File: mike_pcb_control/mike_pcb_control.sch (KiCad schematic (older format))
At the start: 5 parts, among them J1 Conn_01x06_Male, J4 Raspberry_Pi_2_3, U3 LLC-4channel, U4 Adafruit_Feather_Pinout

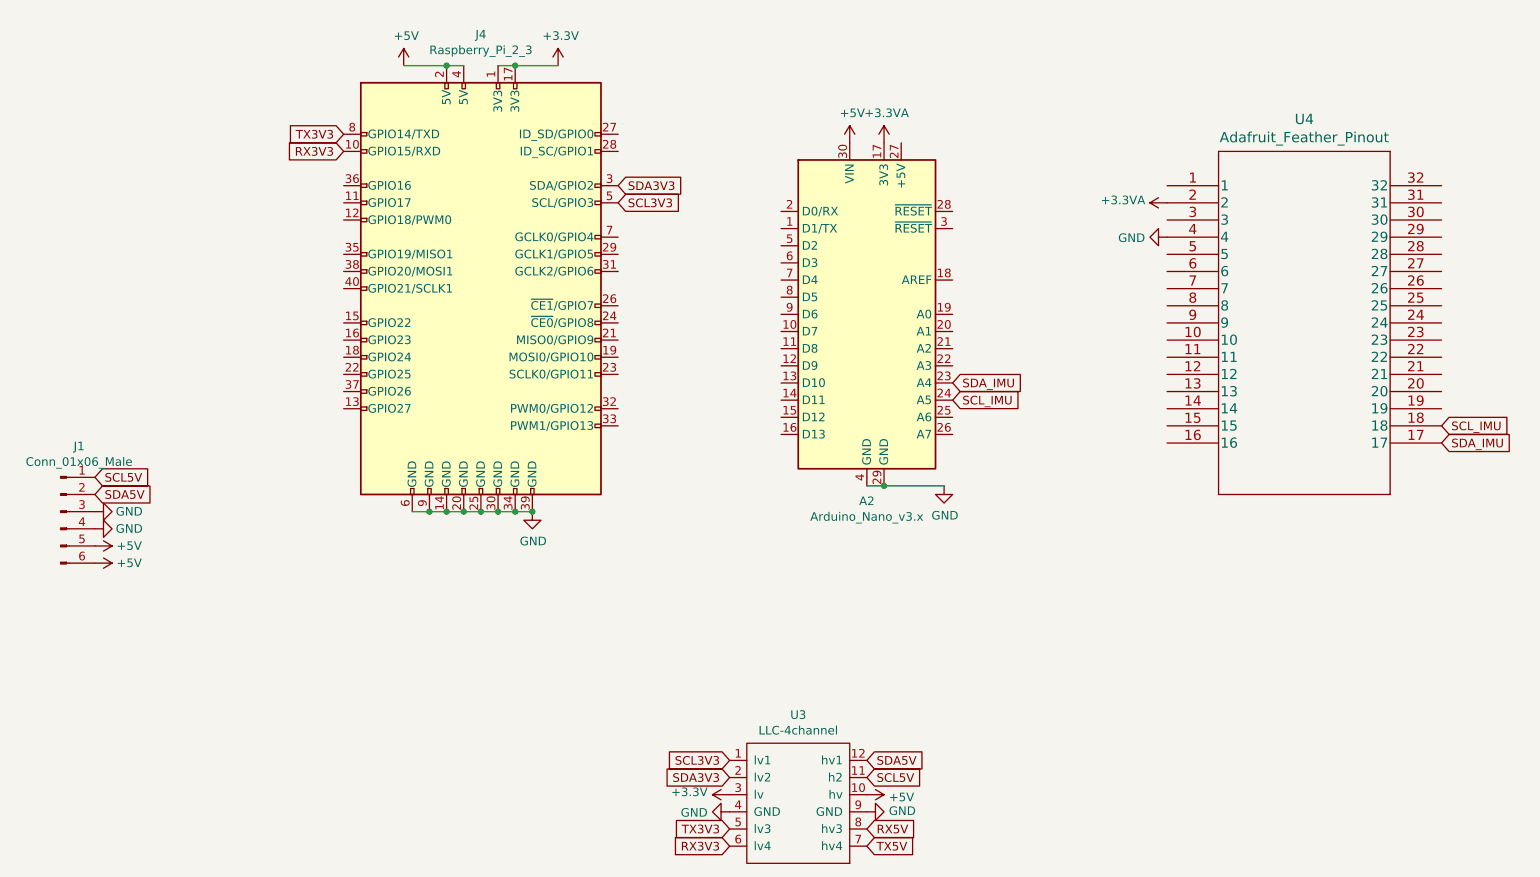
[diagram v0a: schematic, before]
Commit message: Updating the design files
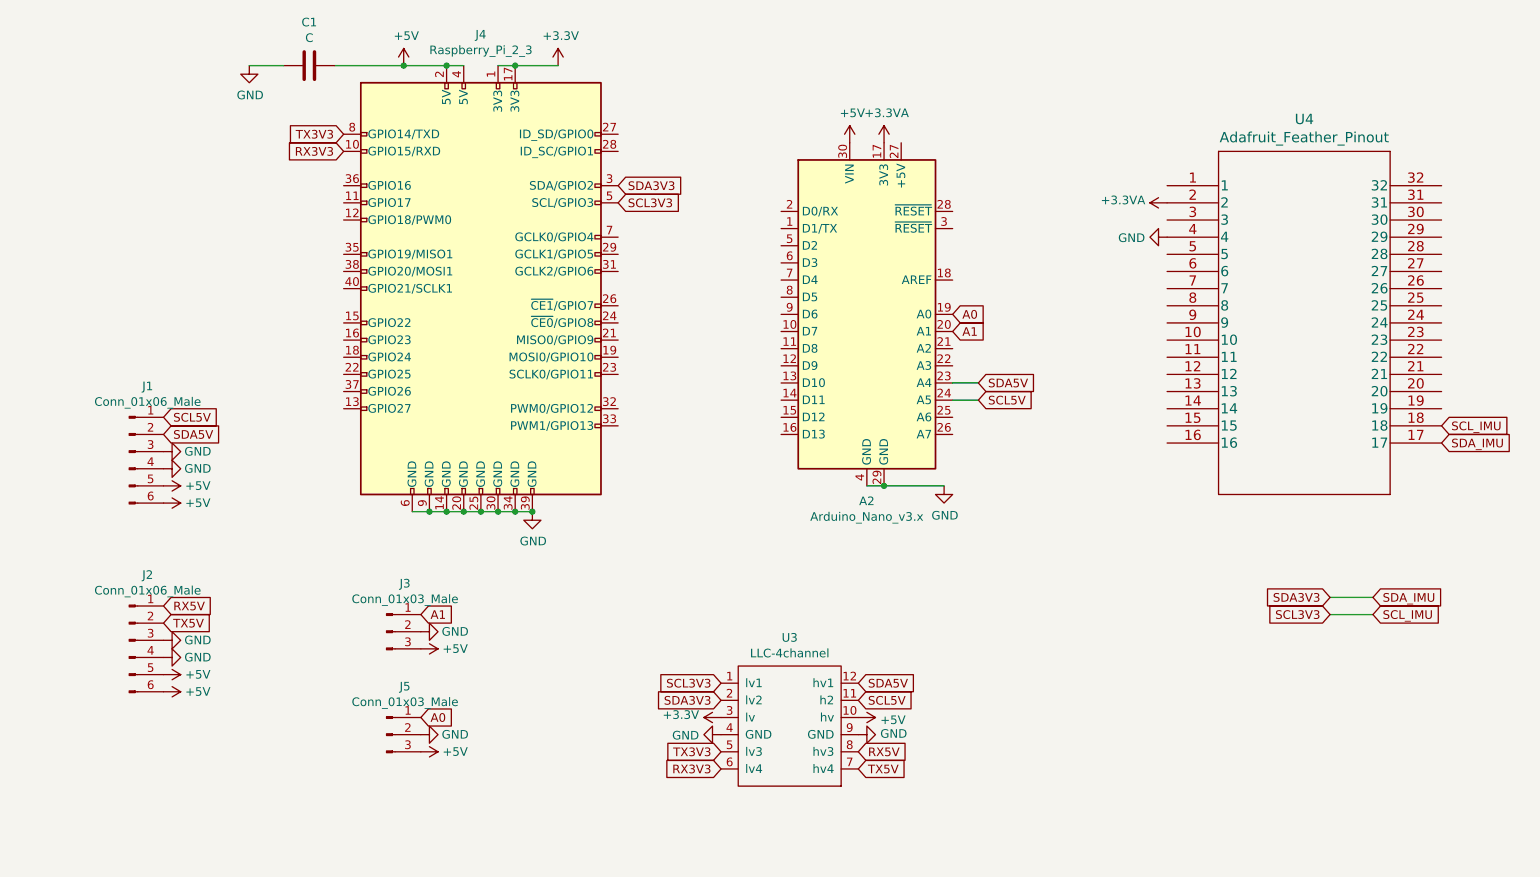
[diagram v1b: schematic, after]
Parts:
- added C1: C, Capacitor_THT:C_Radial_D8.0mm_H7.0mm_P3.50mm, symbol Device:C
- added J2: Conn_01x06_Male, Connector_PinHeader_2.54mm:PinHeader_1x06_P2.54mm_Vertical, symbol Connector:Conn_01x06_Male
- added J3, J5: Conn_01x03_Male, Connector_PinHeader_2.54mm:PinHeader_1x03_P2.54mm_Vertical, symbol Connector:Conn_01x03_Male
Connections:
- net +5V: now also C1.1, J2.5 (Pin_5), J2.6 (Pin_6), J3.3 (Pin_3), J5.3 (Pin_3)
- net GND: now also C1.2, J2.3 (Pin_3), J2.4 (Pin_4), J3.2 (Pin_2), J5.2 (Pin_2)
- net RX5V: now also J2.1 (Pin_1)
- net SCL3V3: now also U4.18
- net SCL5V: now also A2.24 (A5)
- net SDA3V3: now also U4.17
- net SDA5V: now also A2.23 (A4)
- net TX5V: now also J2.2 (Pin_2)
- net A0: now reaches A2.19 (A0)
- net A0: now also J5.1 (Pin_1)
- net A1: now reaches A2.20 (A1)
- net A1: now also J3.1 (Pin_1)
- removed net SCL_IMU: A2.24 (A5), U4.18
- removed net SDA_IMU: A2.23 (A4), U4.17
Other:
- moved on the sheet: J1, U3
